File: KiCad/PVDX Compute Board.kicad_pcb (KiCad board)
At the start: 2 copper layers, 66.5 x 64 mm, 43 parts, among them IC1 MIC5350-SGYMT-TR, J1 Conn_02x06_Counter_Clockwise, J2 USB_C_Receptacle_USB2.0_14P, J3 Conn_01x07, J4 Conn_01x06, U1 EM008LX, U2 EM008LX, U3 EM008LX, U4 SAMD51, X1 2x5 0.05" SWD

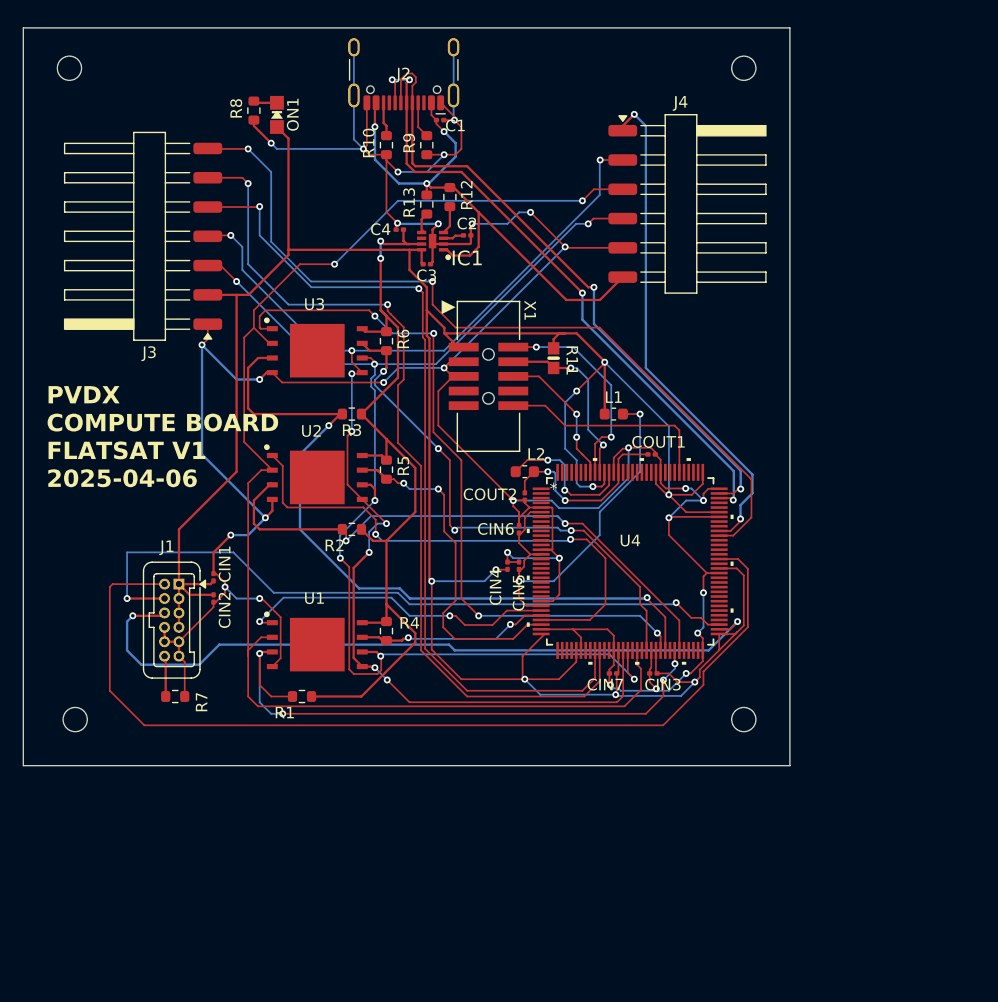
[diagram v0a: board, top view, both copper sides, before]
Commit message: update draft to 11/13 version
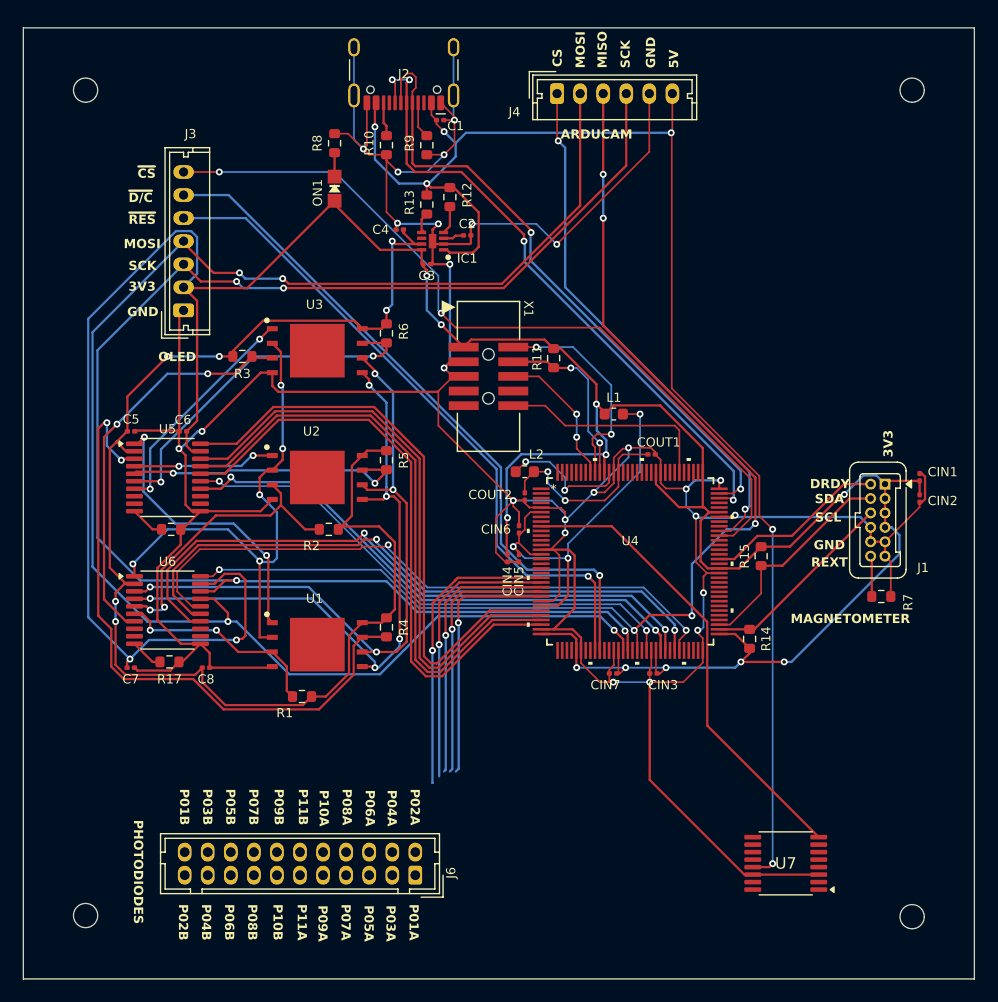
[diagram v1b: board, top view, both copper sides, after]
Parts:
- added C5: 0.1 uF, Capacitor_SMD:C_0201_0603Metric, F.Cu at (148.3, 54.5)
- added C6: 0.1 uF, Capacitor_SMD:C_0201_0603Metric, F.Cu at (152.8, 54.5)
- added C7: 0.1 uF, Capacitor_SMD:C_0201_0603Metric, F.Cu at (148.3, 75.0)
- added C8: 0.1 uF, Capacitor_SMD:C_0201_0603Metric, F.Cu at (154.8, 75.0)
- added J6: Conn_02x11_Counter_Clockwise, Connector_Hirose:Hirose_DF11-22DP-2DSA_2x11_P2.00mm_Vertical, F.Cu at (173.0, 93.0)
- added R14: 10K, Resistor_SMD:R_0603_1608Metric, F.Cu at (202.0, 72.5)
- added R15: 10K, Resistor_SMD:R_0603_1608Metric, F.Cu at (203.0, 65.3)
- added R16: 10K, Resistor_SMD:R_0603_1608Metric, F.Cu at (151.8, 63.0)
- added R17: 10K, Resistor_SMD:R_0603_1608Metric, F.Cu at (151.7, 74.5)
- added U5: TXS0108EPW, Package_SO:TSSOP-20_4.4x6.5mm_P0.65mm, F.Cu at (151.5, 58.5)
- added U6: TXS0108EPW, Package_SO:TSSOP-20_4.4x6.5mm_P0.65mm, F.Cu at (151.5, 70.0)
- added U7: TMUX1108PW, Package_SO:TSSOP-16_4.4x5mm_P0.65mm, F.Cu at (205.1, 92.0)
- CIN1, CIN4: value 10 μF -> 10 uF
- CIN2: value 0.1 μF -> 0.1 uF
- J3: footprint Connector_Harwin:Harwin_M20-89007xx_1x07_P2.54mm_Horizontal -> Connector_Molex:Molex_Micro-Latch_53253-0770_1x07_P2.00mm_Vertical
- J4: footprint Connector_Harwin:Harwin_M20-89006xx_1x06_P2.54mm_Horizontal -> Connector_Molex:Molex_Micro-Latch_53253-0670_1x06_P2.00mm_Vertical
- L1: value 10 μH -> 10 uH
- R11: footprint Adafruit Grand Central M4 Express rev B:0603-NO -> Resistor_SMD:R_0603_1608Metric
- moved CIN1 61.9 mm to (216.8, 58.5)
- moved CIN2 61.9 mm to (216.8, 60.3)
- moved J1 61.9 mm to (213.8, 59.1)
- moved R7 61.9 mm to (213.4, 68.8)
- moved H3 22.5 mm to (216.1, 96.6)
- moved H4 17.0 mm to (144.4, 96.5)
- moved J4 14.8 mm to (185.3, 25.2)
- moved H2 14.7 mm to (216.1, 24.9)
- moved R3 10.7 mm to (158.0, 48.0), turned to 0 degrees
- moved ON1 8.12 mm to (166.0, 33.5)
- moved R8 7.55 mm to (166.0, 29.5), turned to -90 degrees
- moved J3 7.28 mm to (152.9, 44.0), turned to 90 degrees
- moved H1 2.36 mm to (144.4, 24.9)
- moved R2 2.00 mm to (165.5, 63.0)
- moved R5 0.83 mm to (170.5, 57.0), turned to 90 degrees
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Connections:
- net 3.3V renamed 3V3
- C4 pad 1: 1.8V -> 1V8
- IC1 pad 7: 1.8V -> 1V8
- R1 pad 1: 1.8V -> 1V8
- R1 pad 2: PC14 -> PC14 1V8
- R2 pad 1: 1.8V -> 1V8
- R2 pad 2: PC15 -> PC15 1V8
- R3 pad 1: 1.8V -> 1V8
- R3 pad 2: PC12 -> PC12 1V8
- R4 pad 1: 1.8V -> PC05 1V8
- R4 pad 2: PC05 -> 1V8
- R5 pad 1: 1.8V -> PC07 1V8
- R5 pad 2: PC07 -> 1V8
- R6 pad 1: 1.8V -> PC10 1V8
- R6 pad 2: PC10 -> 1V8
- U1 pad 1: PC04 -> PC04 1V8
- U1 pad 2: PD11 (MISO) -> PD11 (MISO) 1V8
- U1 pad 3: PC14 -> PC14 1V8
- U1 pad 5: PD08 (MOSI) -> PD08 (MOSI) 1V8
- U1 pad 6: PD09 (SCK) -> PD09 (SCK) 1V8
- U1 pad 7: PC05 -> PC05 1V8
- U1 pad 8: 1.8V -> 1V8
- U2 pad 1: PC06 -> PC06 1V8
- U2 pad 2: PD11 (MISO) -> PD11 (MISO) 1V8
- U2 pad 3: PC15 -> PC15 1V8
- U2 pad 5: PD08 (MOSI) -> PD08 (MOSI) 1V8
- U2 pad 6: PD09 (SCK) -> PD09 (SCK) 1V8
- U2 pad 7: PC07 -> PC07 1V8
- U2 pad 8: 1.8V -> 1V8
- U3 pad 1: PC11 -> PC11 1V8
- U3 pad 2: PD11 (MISO) -> PD11 (MISO) 1V8
- U3 pad 3: PC12 -> PC12 1V8
- U3 pad 5: PD08 (MOSI) -> PD08 (MOSI) 1V8
- U3 pad 6: PD09 (SCK) -> PD09 (SCK) 1V8
- U3 pad 7: PC10 -> PC10 1V8
- U3 pad 8: 1.8V -> 1V8
- U4 pad 10: unconnected-(U4B-PA03/AIN01-Pad10) -> AIN01
- U4 pad 125: unconnected-(U4C-PB00/AIN12-Pad125) -> AIN12
- U4 pad 126: unconnected-(U4C-PB01/AIN13-Pad126) -> AIN13
- U4 pad 127: unconnected-(U4C-PB02/AIN14-Pad127) -> AIN14
- U4 pad 128: unconnected-(U4C-PB03/AIN15-Pad128) -> AIN15
- U4 pad 19: unconnected-(U4C-PB08/AIN02-Pad19) -> AIN02
- U4 pad 20: unconnected-(U4C-PB09/AIN03-Pad20) -> AIN03
- U4 pad 21: unconnected-(U4B-PA04/AIN04-Pad21) -> AIN04
- U4 pad 22: unconnected-(U4B-PA05/AIN05-Pad22) -> AIN05
- U4 pad 23: unconnected-(U4B-PA06/AIN06-Pad23) -> AIN06
- U4 pad 24: unconnected-(U4B-PA07/AIN07-Pad24) -> AIN07
- U4 pad 33: unconnected-(U4B-PA08/AIN08-Pad33) -> AIN08
- U4 pad 34: unconnected-(U4B-PA09/AIN09-Pad34) -> AIN09
- U4 pad 35: unconnected-(U4B-PA10/AIN10-Pad35) -> AIN10
- U4 pad 36: unconnected-(U4B-PA11/AIN11-Pad36) -> AIN11
- U4 pad 9: unconnected-(U4B-PA02/AIN00-Pad9) -> AIN00
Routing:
- net 1V8: track 0.00 -> 118.9 mm, vias 0 -> 6
- net 5V: track 48.3 -> 123.1 mm, vias 3 -> 6
- net 1.8V: track 71.7 -> 0.00 mm, vias 2 -> 0
- net GND: track 300.0 -> 370.9 mm, vias 30 -> 25
- net PD21: track 82.2 -> 15.8 mm
- net PD09 (SCK) 1V8: track 0.00 -> 56.8 mm, vias 0 -> 4
- net PC05 1V8: track 0.00 -> 56.5 mm, vias 0 -> 2
- net PD08 (MOSI) 1V8: track 0.00 -> 55.4 mm, vias 0 -> 5
- net PA16 (SCL): track 63.4 -> 17.3 mm, vias 2 -> 0
- net PD11 (MISO) 1V8: track 0.00 -> 44.6 mm, vias 0 -> 5
- net PA17 (SDA): track 62.8 -> 20.6 mm, vias 2 -> 0
- net AIN00: track 0.00 -> 40.5 mm
- net PC05: track 16.9 -> 52.5 mm, vias 2 -> 0
- net PC12 1V8: track 0.00 -> 35.1 mm, vias 0 -> 2
- net PC10 1V8: track 0.00 -> 31.2 mm, vias 0 -> 2
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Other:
- board size 66.5 x 64 mm -> 82.5 x 82.5 mm
- board text added: "3V3"
- board text added: "5V"
- board text added: "ARDUCAM"
- board text added: "CS"
- board text added: "DRDY"
- board text added: "GND"
- board text added: "MAGNETOMETER"
- board text added: "MISO"
- board text added: "MOSI"
- board text added: "OLED"
- board text added: "P01A"
- board text added: "P01B"
- board text added: "P02A"
- board text added: "P02B"
- board text added: "P03A"
- board text added: "P03B"
- board text added: "P04A"
- board text added: "P04B"
- board text added: "P05A"
- board text added: "P05B"
- board text added: "P06A"
- board text added: "P06B"
- board text added: "P07A"
- board text added: "P07B"
- board text added: "P08A"
- board text added: "P08B"
- board text added: "P09A"
- board text added: "P09B"
- board text added: "P10A"
- board text added: "P10B"
- board text added: "P11A"
- board text added: "P11B"
- board text added: "PHOTODIODES"
- board text added: "REXT"
- board text added: "SCK"
- board text added: "SCL"
- board text added: "SDA"
- board text added: "~{CS}"
- board text added: "~{D/C}"
- board text added: "~{RES}"
- board text removed: "PVDX COMPUTE BOARD FLATSAT V1 2025-04-06"
